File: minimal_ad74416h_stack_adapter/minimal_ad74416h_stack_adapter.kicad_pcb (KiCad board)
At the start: 4 copper layers, 45.7 x 53.3 mm, 5 parts, among them J1 FW-33-03-G-D-085-155, J2 CLP-133-02-G-D-BE, J3 CLP-133-02-G-D-BE, J4 CLP-133-02-G-D-BE, J5 CLP-133-02-G-D-BE

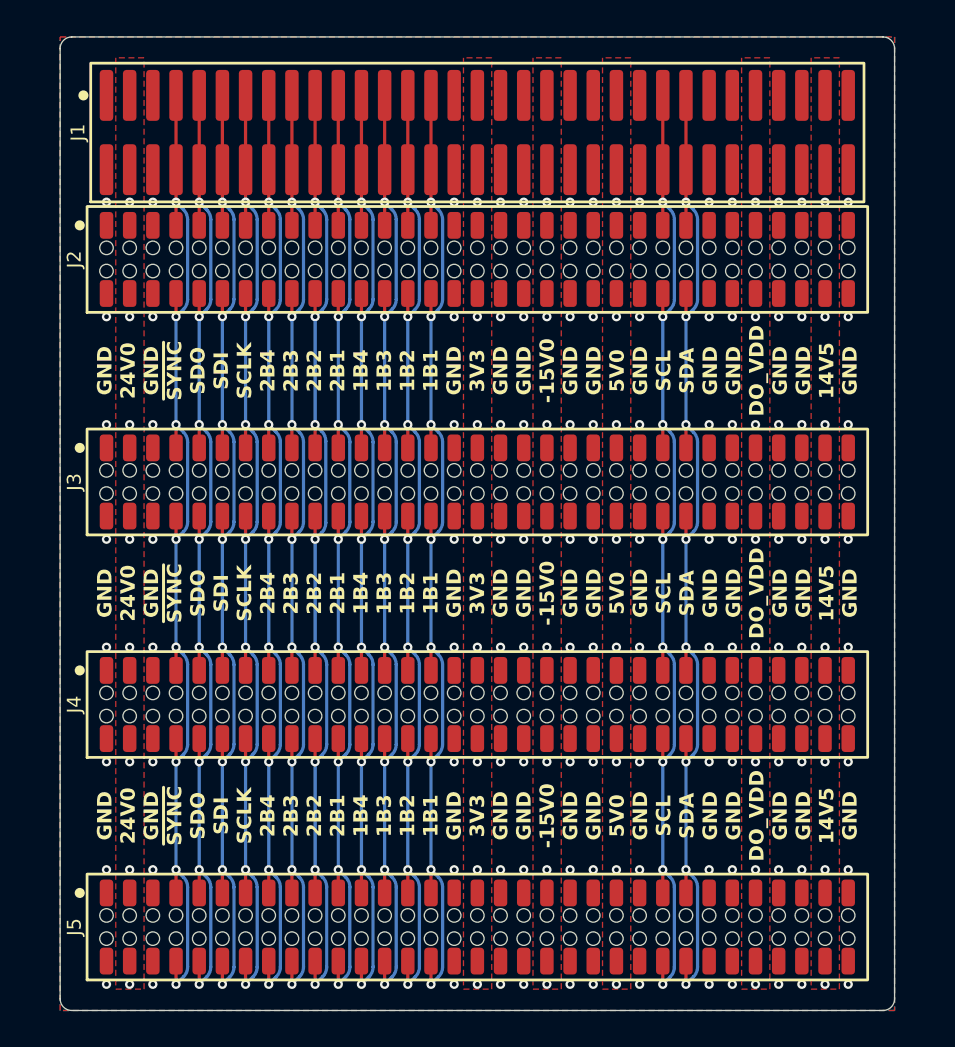
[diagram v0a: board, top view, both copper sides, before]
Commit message: backup
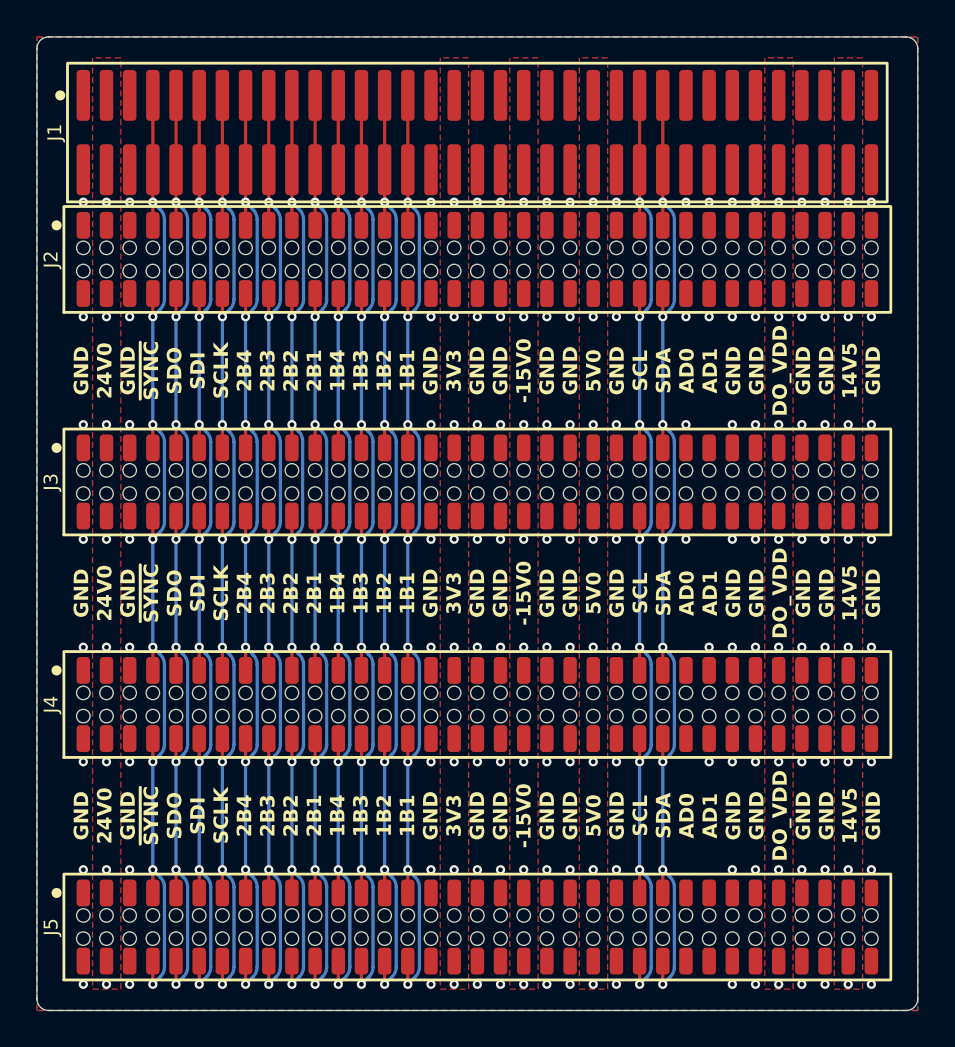
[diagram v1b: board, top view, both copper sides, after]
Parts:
- J1: renamed from J4; value CLP-133-02-G-D-BE -> FW-35-03-G-D-085-155; footprint connector_footprints:CLP-133-02-G-D-BE -> connector_footprints:FW-35-03-G-D-085-155
- J2, J3, J5: value CLP-133-02-G-D-BE -> CLP-135-02-G-D-BE; footprint connector_footprints:CLP-133-02-G-D-BE -> connector_footprints:CLP-135-02-G-D-BE
- J4: renamed from J1; value FW-33-03-G-D-085-155 -> CLP-135-02-G-D-BE; footprint connector_footprints:FW-33-03-G-D-085-155 -> connector_footprints:CLP-135-02-G-D-BE
- moved J1 31.3 mm to (139.7, 99.2)
- moved J4 31.3 mm to (139.7, 130.6)
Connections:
- J1 pad 53: GNDA -> unconnected-(J1-Pad53)
- J1 pad 54: GNDA -> unconnected-(J1-Pad54)
- J1 pad 55: GNDA -> unconnected-(J1-Pad55)
- J1 pad 56: GNDA -> unconnected-(J1-Pad56)
- J1 pad 57: /DO_VDD -> GNDA
- J1 pad 58: /DO_VDD -> GNDA
- J1 pad 61: GNDA -> /DO_VDD
- J1 pad 62: GNDA -> /DO_VDD
- J1 pad 63: /14V5 -> GNDA
- J1 pad 64: /14V5 -> GNDA
- J2 pad 57: /DO_VDD -> GNDA
- J2 pad 58: /DO_VDD -> GNDA
- J2 pad 61: GNDA -> /DO_VDD
- J2 pad 62: GNDA -> /DO_VDD
- J2 pad 63: /14V5 -> GNDA
- J2 pad 64: /14V5 -> GNDA
- J3 pad 55: GNDA -> unconnected-(J3-Pad55)
- J3 pad 56: GNDA -> unconnected-(J3-Pad56)
- J3 pad 57: /DO_VDD -> GNDA
- J3 pad 58: /DO_VDD -> GNDA
- J3 pad 61: GNDA -> /DO_VDD
- J3 pad 62: GNDA -> /DO_VDD
- J3 pad 63: /14V5 -> GNDA
- J3 pad 64: /14V5 -> GNDA
- J4 pad 53: GNDA -> unconnected-(J4-Pad53)
- J4 pad 54: GNDA -> unconnected-(J4-Pad54)
- J4 pad 57: /DO_VDD -> GNDA
- J4 pad 58: /DO_VDD -> GNDA
- J4 pad 61: GNDA -> /DO_VDD
- J4 pad 62: GNDA -> /DO_VDD
- J4 pad 63: /14V5 -> GNDA
- J4 pad 64: /14V5 -> GNDA
- J5 pad 53: GNDA -> unconnected-(J5-Pad53)
- J5 pad 54: GNDA -> unconnected-(J5-Pad54)
- J5 pad 55: GNDA -> unconnected-(J5-Pad55)
- J5 pad 56: GNDA -> unconnected-(J5-Pad56)
- J5 pad 57: /DO_VDD -> GNDA
- J5 pad 58: /DO_VDD -> GNDA
- J5 pad 61: GNDA -> /DO_VDD
- J5 pad 62: GNDA -> /DO_VDD
- J5 pad 63: /14V5 -> GNDA
- J5 pad 64: /14V5 -> GNDA
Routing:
- net GNDA: vias 104 -> 112
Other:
- board size 45.7 x 53.3 mm -> 48.3 x 53.3 mm
- board text added: "GND 24V0 GND ~{SYNC} SDO SDI SCLK 2B4 2B3 2B2 2B1 1B4 1B3 1B2 1B1 GND 3V3 GND GND -15V0 GND GND 5V0 GND SCL SDA AD0 AD1 GND GND DO_VDD GND GND 14V5 GND"
- board text removed: "GND 24V0 GND ~{SYNC} SDO SDI SCLK 2B4 2B3 2B2 2B1 1B4 1B3 1B2 1B1 GND 3V3 GND GND -15V0 GND GND 5V0 GND SCL SDA GND GND DO_VDD GND GND 14V5 GND"
